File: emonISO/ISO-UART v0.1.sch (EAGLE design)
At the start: 24 parts

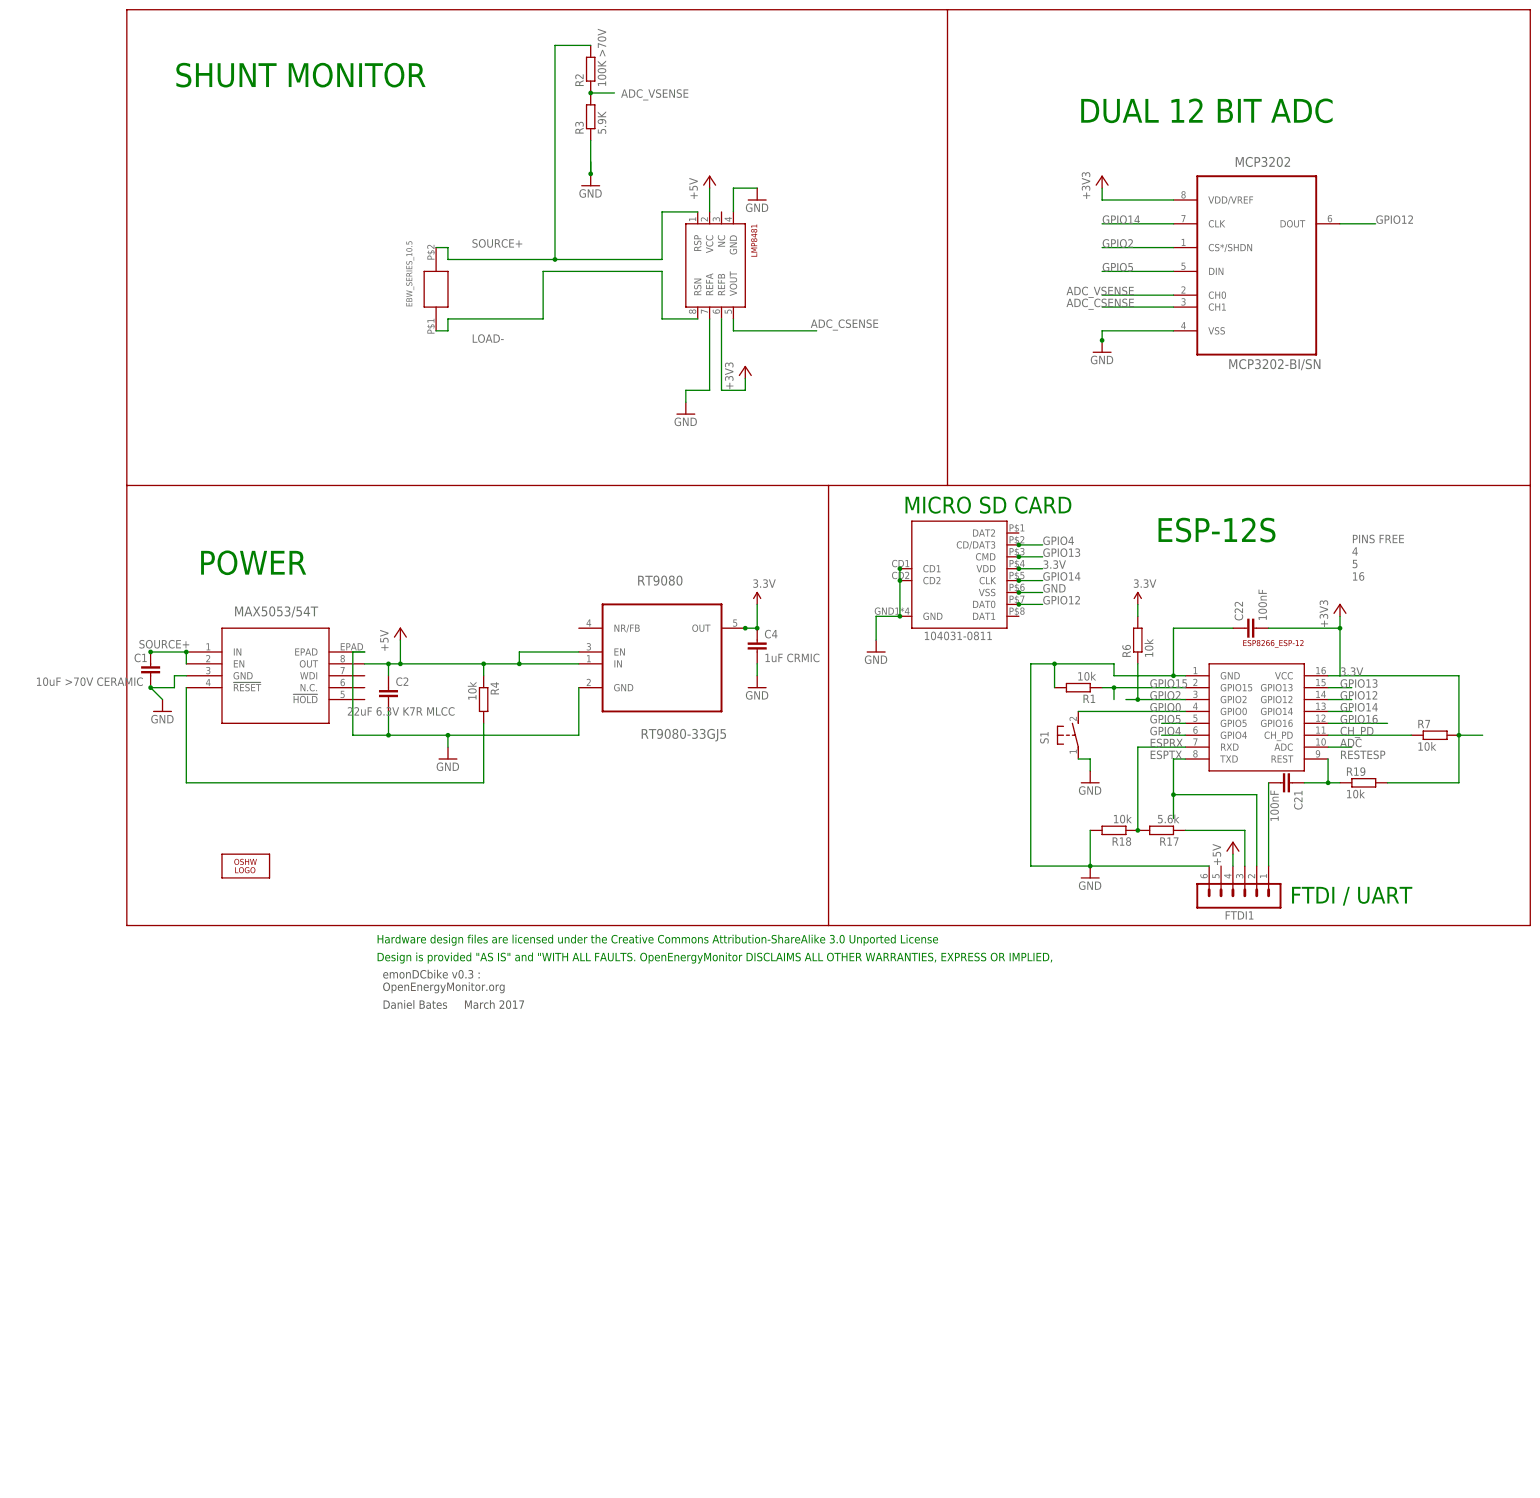
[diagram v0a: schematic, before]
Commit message: commit
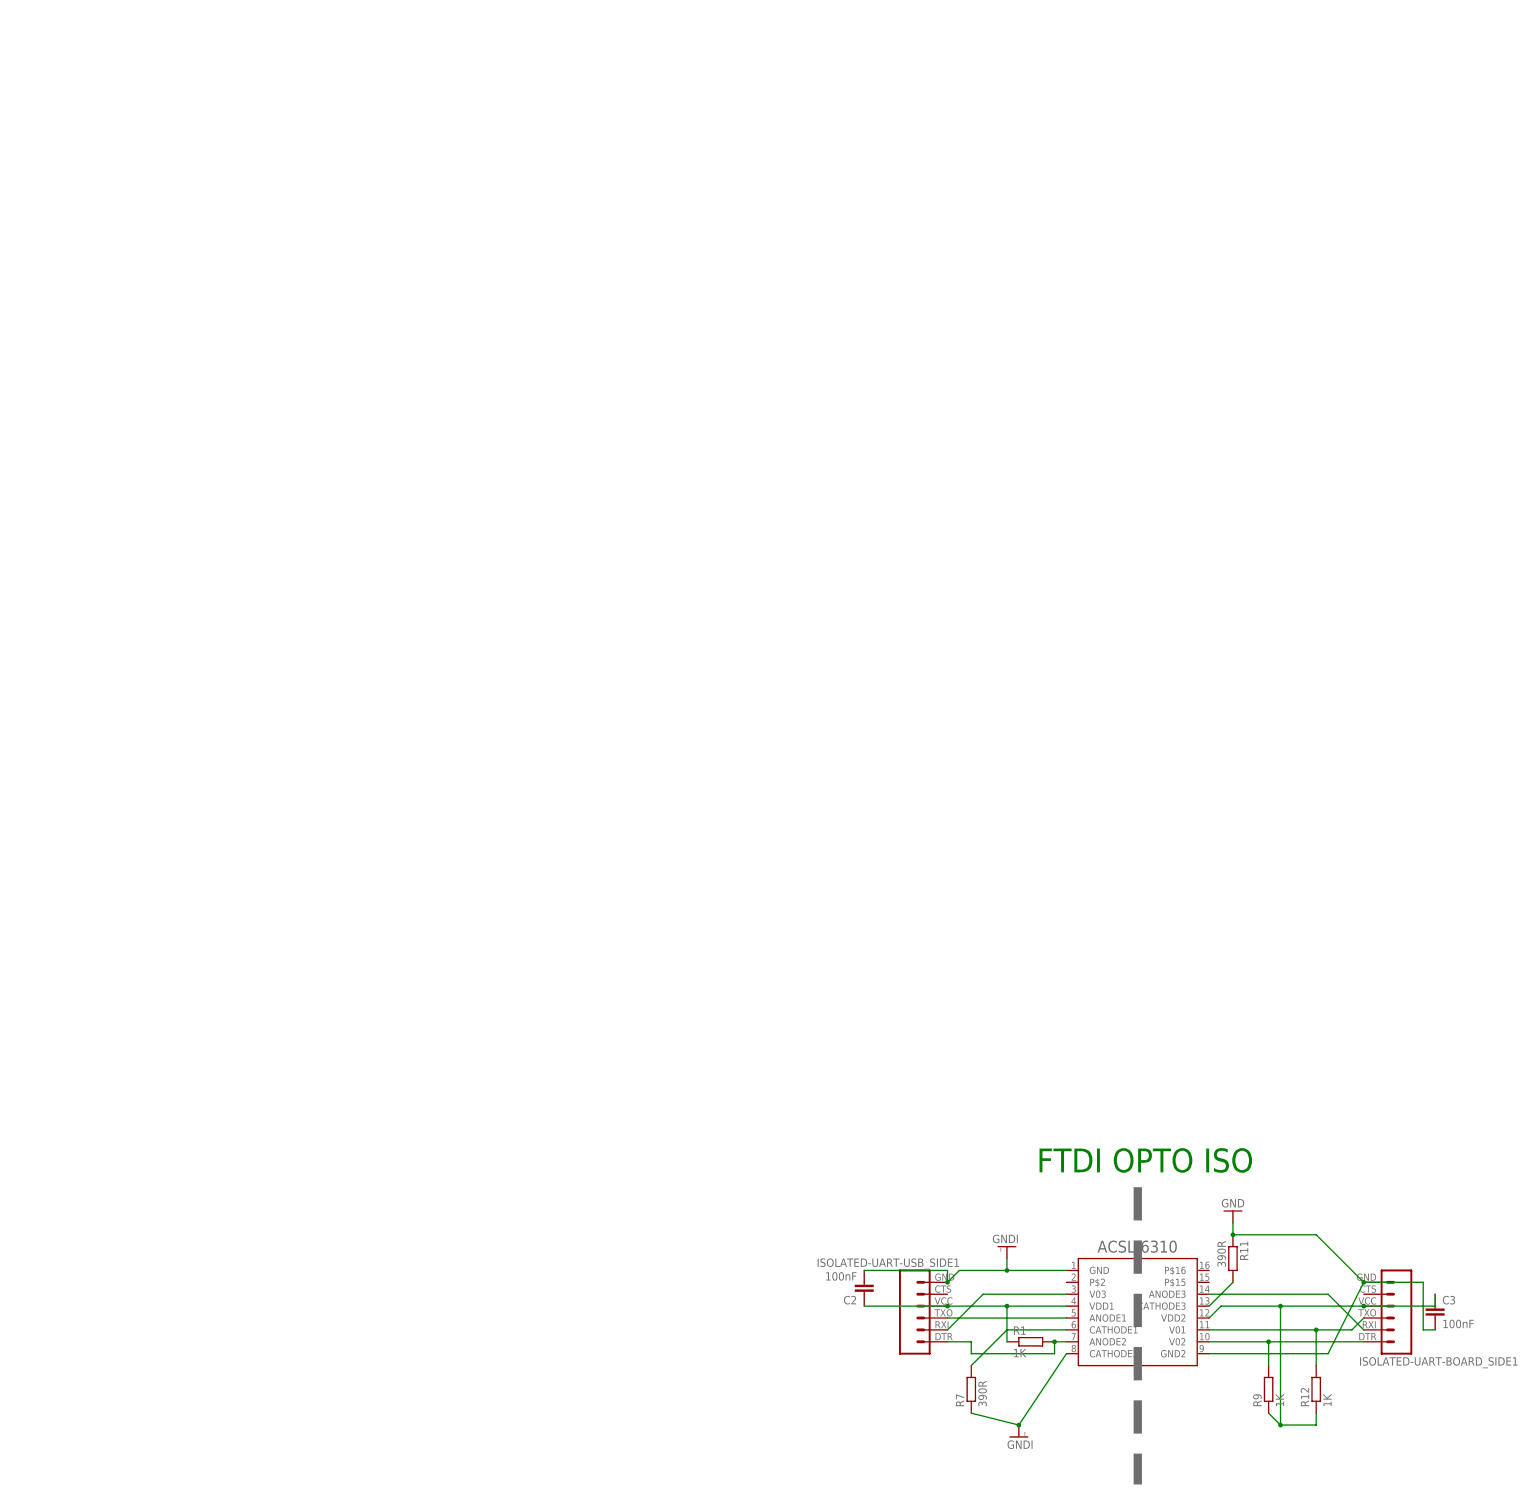
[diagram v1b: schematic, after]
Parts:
- removed C1: 10uF >70V CERAMIC, rcl:C-EUC0603
- removed C21, C22: 100nF, rcl:C-EUC0603
- removed C4: 1uF CRMIC, rcl:C-EUC0603
- removed EBW_SERIES_10.5: EBW_SERIES_10.5MM, EBW series shunt:EBW_SERIES_10.5MM
- removed ESP-12: ESP8266_ESP-12, ESP8266-ESP12:ESP8266_ESP-12
- removed FTDI1: FTDI-ESP, JeeLabs:MA06-1
- removed LMP8481: LMP8481-H, lmp8481b:LMP8481LMP8481-H
- removed LOGO1: OSHW_LOGO_6MILX0200-NT, ohw-logo:OSHW_LOGO_6MILX0200-NT
- removed MAX5053: MAX5023TASA-T21-0111D_SBE-14-L, MAX5053:MAX5023TASA-T21-0111D_SBE-14-L
- removed MCP3202: MCP3202-BI/SN, Microchip-MCP3202-BI_SN:MCP3202-BI/SN
- removed R17: 5.6k, rcl:R-EU_R0603
- removed R18, R19, R4, R6: 10k, rcl:R-EU_R0603
- removed R2: 100K >70V, rcl:R-EU_R0603
- removed R3: 5.9K, rcl:R-EU_R0603
- removed RT9080: RT9080-33GJ5, TSOT-23-5 REGULATOR 3.3v:RT9080-33GJ5
- removed S1: DTSM-3, switch-tact:DTSM-3
- removed U$1: MOLEX_104031-0811, MOLEX MICRO SD [exposed pins]:MOLEX_104031-0811
- added ACSL-6310: ACSL-6310, PACKAGES FOR TEST BOARDS:ACSL-6310
- added C3: 100nF, rcl:C-EUC0603
- added ISOLATED-UART-BOARD_SIDE1, ISOLATED-UART-USB_SIDE1: 2211S-06G, SparkFun:FTDI_BASICPTH
- added R11: 390R, rcl:R-EU_R0603
- added R12, R9: 1K, rcl:R-EU_R0603
- C2: value 22uF 6.3V K7R MLCC -> 100nF; device rcl:C-EUC1206 -> rcl:C-EUC0603
- R1: value 10k -> 1K
- R7: value 10k -> 390R
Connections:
- removed net +5V: C2.1, FTDI1.4, MAX5053.OUT, R4.1, RT9080.EN, RT9080.IN
- removed net 3.3V: C22.2, C4.1, ESP-12.VCC, LMP8481.REFB, MCP3202.VDD/VREF, R19.2, R6.2, R7.2, RT9080.OUT, U$1.VDD
- removed net ADC: ESP-12.ADC
- removed net ADC_CSENSE: LMP8481.VOUT, MCP3202.CH1
- removed net ADC_VSENSE: MCP3202.CH0, R2.1, R3.2
- removed net CH_PD: ESP-12.CH_PD, R7.1
- removed net ESPRX: ESP-12.RXD, R17.2, R18.1
- removed net ESPTX: ESP-12.TXD, FTDI1.2
- removed net GPIO0: ESP-12.GPIO0, S1.2
- removed net GPIO12: ESP-12.GPIO12, MCP3202.DOUT, U$1.DAT0
- removed net GPIO13: ESP-12.GPIO13, U$1.CMD
- removed net GPIO14: ESP-12.GPIO14, MCP3202.CLK, U$1.CLK
- removed net GPIO15: ESP-12.GPIO15, R1.1
- removed net GPIO16: ESP-12.GPIO16
- removed net GPIO2: ESP-12.GPIO2, MCP3202.CS*/SHDN, R6.1
- removed net GPIO4: ESP-12.GPIO4, U$1.CD/DAT3
- removed net GPIO5: ESP-12.GPIO5, MCP3202.DIN
- removed net LOAD-: EBW_SERIES_10.5.P$1, LMP8481.RSN
- removed net N$1: MAX5053.!RESET, R4.2
- removed net N$36: FTDI1.3, R17.1
- removed net RESTESP: C21.1, ESP-12.REST, R19.1
- removed net RST: C21.2, FTDI1.1
- removed net SOURCE+: C1.1, EBW_SERIES_10.5.P$2, LMP8481.RSP, MAX5053.EN, MAX5053.IN, R2.2
- new net GNDI: ACSL-6310.CATHODE2, ACSL-6310.GND, C2.2, ISOLATED-UART-USB_SIDE1.6, R7.1
- new net N$12: ACSL-6310.CATHODE1, R7.2
- new net N$16: ACSL-6310.CATHODE3, R11.2
- new net N$18: ACSL-6310.V01, ISOLATED-UART-BOARD_SIDE1.3, R12.2
- new net N$2: ACSL-6310.VDD1, C2.1, ISOLATED-UART-USB_SIDE1.4, R1.1
- new net N$3: ACSL-6310.ANODE1, ISOLATED-UART-USB_SIDE1.3
- new net N$4: ACSL-6310.ANODE2, ISOLATED-UART-USB_SIDE1.1, R1.2
- new net N$5: ACSL-6310.V03, ISOLATED-UART-USB_SIDE1.2
- new net N$7: ACSL-6310.V02, ISOLATED-UART-BOARD_SIDE1.1, R9.2
- new net N$8: ACSL-6310.VDD2, C3.1, ISOLATED-UART-BOARD_SIDE1.4, R12.1, R9.1
- new net N$9: ACSL-6310.ANODE3, ISOLATED-UART-BOARD_SIDE1.2
- net GND: now also ACSL-6310.GND2, C3.2, ISOLATED-UART-BOARD_SIDE1.6, R11.1; no longer C1.2, C2.2, C22.1, C4.2, ESP-12.GND, FTDI1.6, LMP8481.GND, LMP8481.REFA, MAX5053.EPAD, MAX5053.GND, MCP3202.VSS, R1.2, R18.2, R3.1, RT9080.GND, S1.1, U$1.CD1, U$1.CD2, U$1.GND, U$1.VSS
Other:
- note added: "ACSL-6310"
- note added: "FTDI OPTO ISO"
- note removed: "104031-0811"
- note removed: "DUAL 12 BIT ADC"
- note removed: "Daniel Bates March 2017"
- note removed: "Design is provided "AS IS" and "WITH ALL FAULTS. OpenEnergyMonitor DISCLAIMS ALL OTHER WARRANTIES, EXPRESS OR IMPLIED,"
- note removed: "ESP-12S"
- note removed: "FTDI / UART"
- note removed: "Hardware design files are licensed under the Creative Commons Attribution-ShareAlike 3.0 Unported License"
- note removed: "MICRO SD CARD"
- note removed: "PINS FREE 4 5 16"
- note removed: "POWER"
- note removed: "SHUNT MONITOR"
- note removed: "emonDCbike v0.3 : OpenEnergyMonitor.org"
- moved on the sheet: C2, R1, R7
